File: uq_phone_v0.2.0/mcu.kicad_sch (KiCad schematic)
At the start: 22 parts, among them J6 Conn_ARM_SWD_TagConnect_TC2030, U5 TXB0108RGYR, U6 STM32H733VGHx, U7 TXB0108RGYR

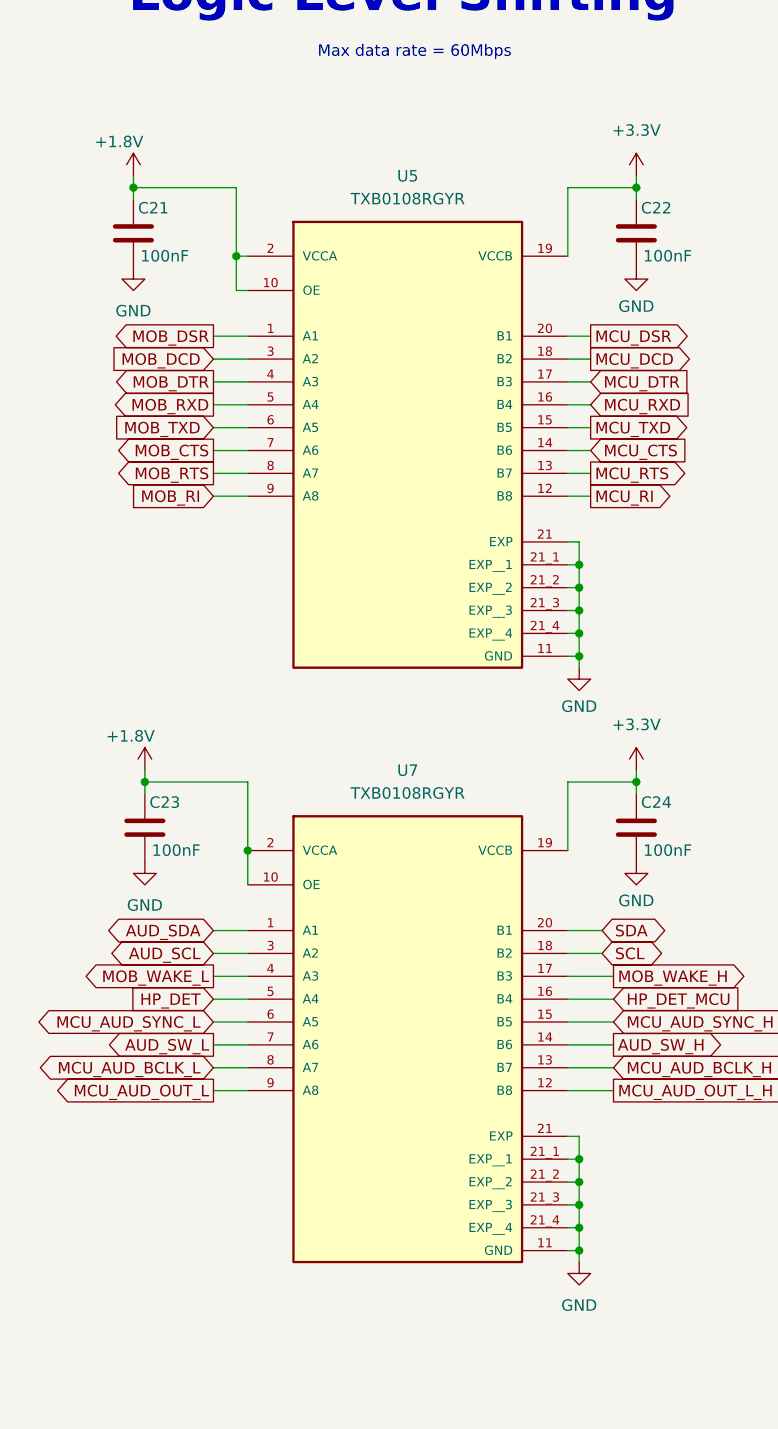
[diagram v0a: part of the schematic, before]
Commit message: Various Changes to footprints and components
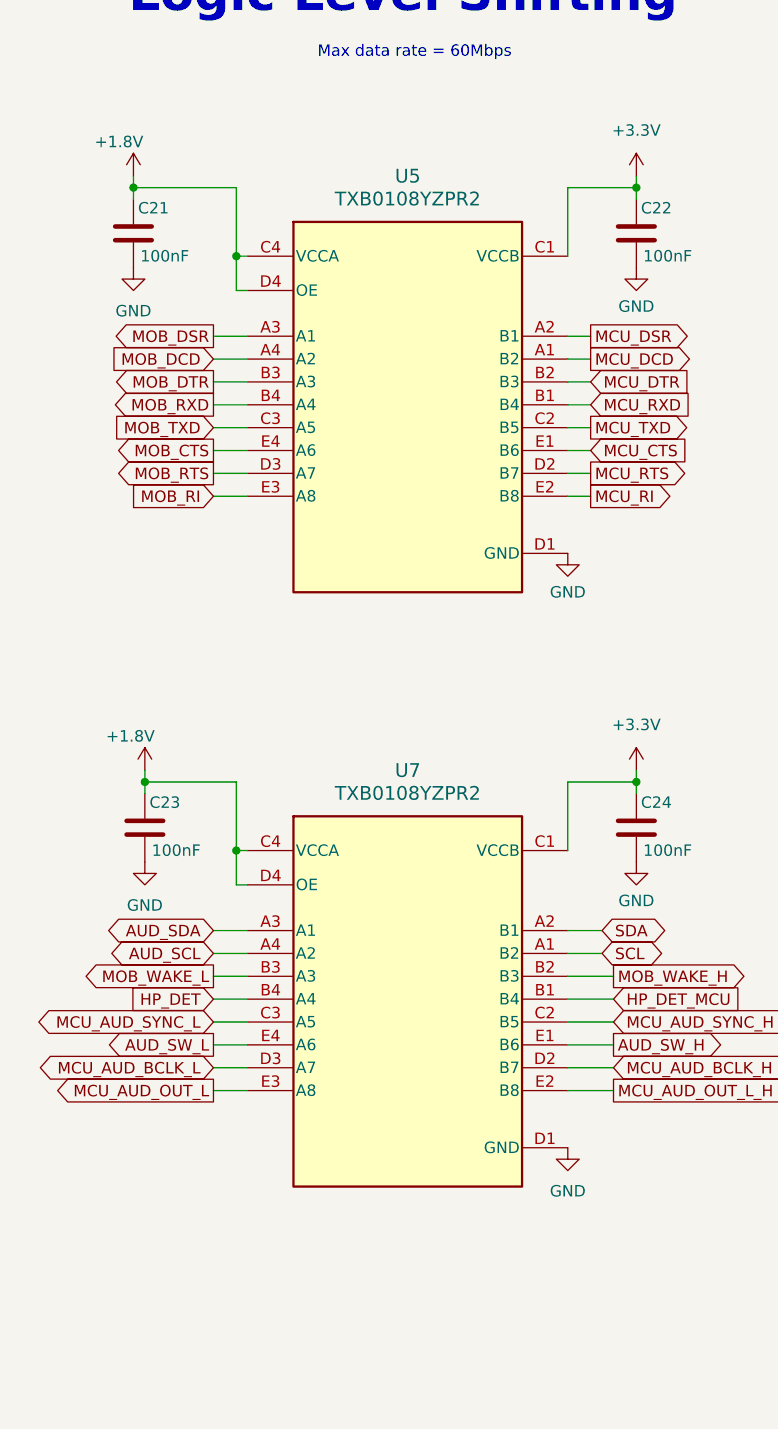
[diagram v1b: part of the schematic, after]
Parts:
- removed U5, U7: TXB0108RGYR, TXB0108RGYR:IC_TXB0108RGYR, symbol TXB0108RGYR:TXB0108RGYR
- added U5, U7: TXB0108YZPR2, TXB0108YZPR2:YZP20, symbol TXB0108YZPR2:TXB0108YZPR2
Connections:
- net +1.8V: now also U5.C4 (VCCA), U5.D4 (OE), U7.C4 (VCCA), U7.D4 (OE)
- net +3.3V: now also U5.C1 (VCCB), U7.C1 (VCCB)
- net AUD_SCL: now also U7.A4 (A2)
- net AUD_SDA: now also U7.A3 (A1)
- net AUD_SW_H: now also U7.E1 (B6)
- net AUD_SW_L: now also U7.E4 (A6)
- net GND: now also U5.D1 (GND), U7.D1 (GND)
- net HP_DET: now also U7.B4 (A4)
- net HP_DET_MCU: now also U7.B1 (B4)
- net MCU_AUD_BCLK_H: now also U7.D2 (B7)
- net MCU_AUD_BCLK_L: now also U7.D3 (A7)
- net MCU_AUD_OUT_L: now also U7.E3 (A8)
- net MCU_AUD_OUT_L_H: now also U7.E2 (B8)
- net MCU_AUD_SYNC_H: now also U7.C2 (B5)
- net MCU_AUD_SYNC_L: now also U7.C3 (A5)
- net MCU_CTS: now also U5.E1 (B6)
- net MCU_DCD: now also U5.A1 (B2)
- net MCU_DSR: now also U5.A2 (B1)
- net MCU_DTR: now also U5.B2 (B3)
- net MCU_RI: now also U5.E2 (B8)
- net MCU_RTS: now also U5.D2 (B7)
- net MCU_RXD: now also U5.B1 (B4)
- net MCU_TXD: now also U5.C2 (B5)
- net MOB_CTS: now also U5.E4 (A6)
- net MOB_DCD: now also U5.A4 (A2)
- net MOB_DSR: now also U5.A3 (A1)
- net MOB_DTR: now also U5.B3 (A3)
- net MOB_RI: now also U5.E3 (A8)
- net MOB_RTS: now also U5.D3 (A7)
- net MOB_RXD: now also U5.B4 (A4)
- net MOB_TXD: now also U5.C3 (A5)
- net MOB_WAKE_H: now also U7.B2 (B3)
- net MOB_WAKE_L: now also U7.B3 (A3)
- net SCL: now also U7.A1 (B2)
- net SDA: now also U7.A2 (B1)
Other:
- title: Power System -> UQ Phone
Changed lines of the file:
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@@
 	(paper "A3")
 	(title_block
-		(title "Power System")
+		(title "UQ Phone")
+		(rev "0.2.0")
 		(company "The University of Queensland")
 	)
